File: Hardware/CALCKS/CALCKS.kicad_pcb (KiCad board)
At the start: 2 copper layers, 68 parts, among them J1 Conn_02x03_Counter_Clockwise, J2 USB_B_Micro, J3 Conn_01x01_Male, J4 Conn_01x01_Male, SW1 SW_Push_Dual, SW10 SW_Push_Dual, SW11 SW_Push_Dual, SW12 SW_Push_Dual, SW13 SW_Push_Dual, SW14 SW_Push_Dual, SW15 SW_Push_Dual, SW16 SW_Push_Dual, SW17 SW_Push_Dual, SW18 SW_Push_Dual, SW19 SW_Push_Dual, SW2 SW_Push_Dual, SW20 SW_Push_Dual, SW21 SW_Push_Dual, SW22 SW_Push_Dual, SW23 SW_Push_Dual, SW24 SW_Push_Dual, SW25 SW_Push_Dual, SW26 SW_Push_Dual, SW27 SW_Push_Dual, SW28 SW_Push_Dual, SW29 SW_Push_Dual, SW3 SW_Push_Dual, SW30 SW_Push_Dual, SW31 SW_Push_Dual, SW32 SW_Push_Dual, SW33 SW_Push_Dual, SW34 SW_Push_Dual, SW35 SW_Push_Dual, SW36 SW_Push_Dual, SW37 SW_Push_Dual, SW38 SW_Push_Dual, SW39 SW_Push_Dual, SW4 SW_Push_Dual, SW40 SW_Push_Dual, SW5 SW_Push_Dual, SW6 SW_Push_Dual, SW7 SW_Push_Dual, SW8 SW_Push_Dual, SW9 SW_Push_Dual, U1 ATmega1284-AU, U2 MCP73831-2-OT, U3 AT24CS64-SSHM, U4 74HC164, Y1 16MHz

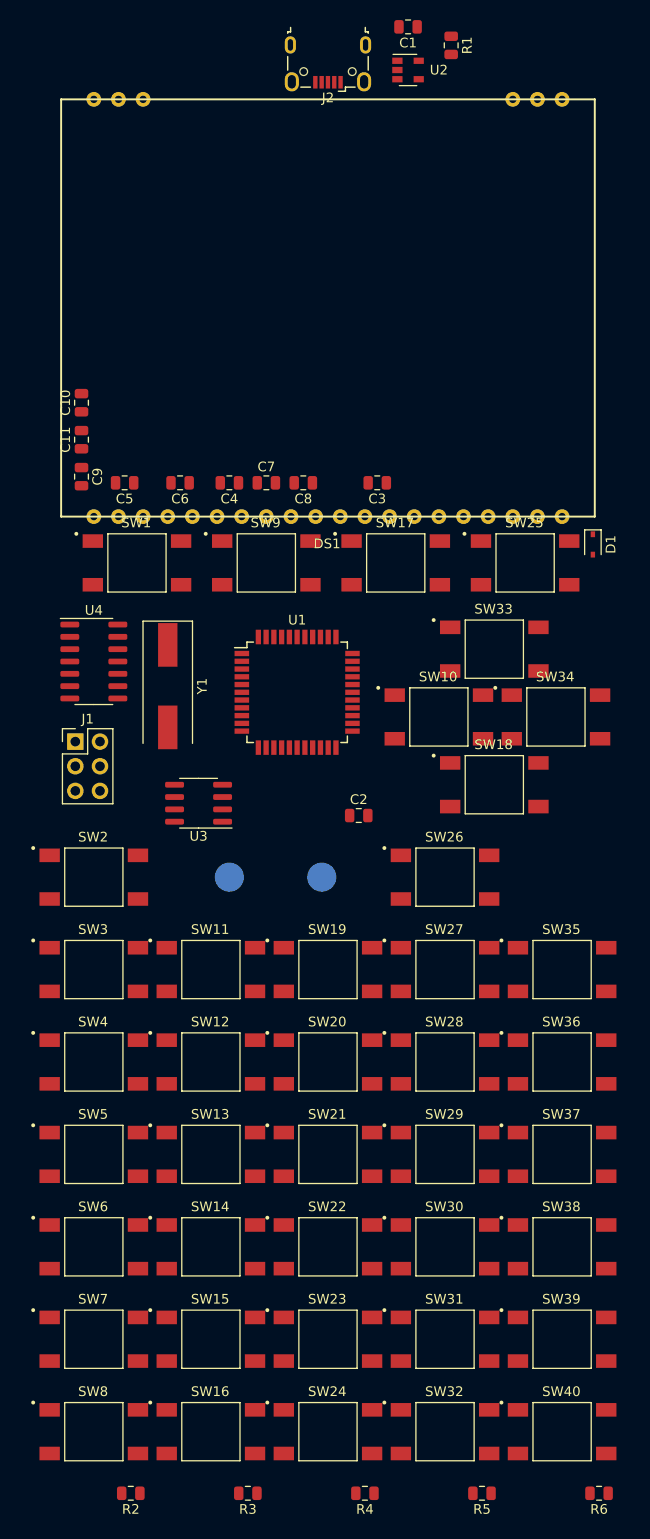
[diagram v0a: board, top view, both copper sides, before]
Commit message: PCB routing
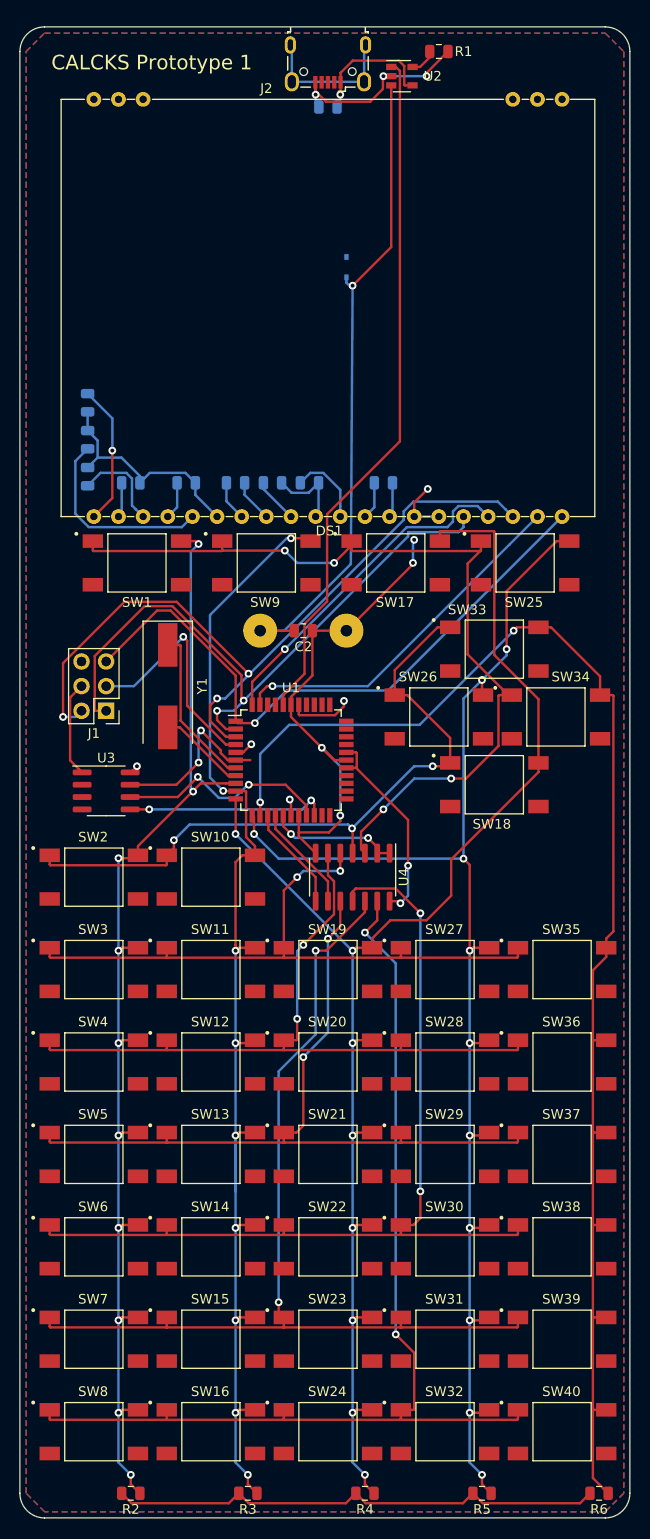
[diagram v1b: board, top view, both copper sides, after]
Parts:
- C1, C10, C11, C3, C4, C5, C6, C7, C8, C9, D1: moved to B.Cu
- J3, J4: footprint TestPoint:TestPoint_Pad_D3.0mm -> Connector_Wire:SolderWirePad_1x01_Drill1.2mm
- moved D1 38.2 mm to (100.3, 50.8)
- moved U4 34.7 mm to (101.0, 113.7), turned to 270 degrees
- moved SW10 28.7 mm to (86.4, 113.7)
- moved J3 28.1 mm to (100.3, 88.3)
- moved J4 26.2 mm to (91.4, 88.3)
- moved C2 19.9 mm to (95.9, 88.3), turned to 180 degrees
- moved SW26 16.5 mm to (109.9, 97.2)
- moved C1 11.7 mm to (98.4, 34.3)
- moved U3 9.61 mm to (75.6, 104.8), turned to 0 degrees
- moved C10 7.65 mm to (73.7, 72.4), turned to 270 degrees
- moved C9 7.65 mm to (73.7, 64.8), turned to 90 degrees
- moved U1 7.01 mm to (94.6, 101.6)
- moved J1 4.49 mm to (75.6, 96.5), turned to 180 degrees
- moved R1 1.42 mm to (109.9, 28.6), turned to 180 degrees
- moved U2 0.90 mm to (106.0, 31.1)
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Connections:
- net Net-(C2-Pad2) renamed +BATT
- C1 pad 2: GND -> Net-(C1-Pad2)
- C10 pad 1: GND -> -BATT
- C11 pad 1: GND -> -BATT
- C2 pad 1: GND -> -BATT
- C3 pad 1: GND -> -BATT
- C5 pad 1: GND -> -BATT
- C6 pad 1: GND -> -BATT
- C9 pad 1: GND -> -BATT
- DS1 pad 26: GND -> -BATT
- DS1 pad 33: GND -> -BATT
- J1 pad 4: GND -> -BATT
- J2 pad 5: GND -> Net-(C1-Pad2)
- J3 pad 1: GND -> -BATT
- R1 pad 1: GND -> Net-(C1-Pad2)
- R2 pad 2: GND -> -BATT
- R3 pad 2: GND -> -BATT
- R4 pad 2: GND -> -BATT
- R5 pad 2: GND -> -BATT
- R6 pad 2: GND -> -BATT
- U1 pad 18: GND -> -BATT
- U1 pad 28: GND -> -BATT
- U1 pad 39: GND -> -BATT
- U1 pad 6: GND -> -BATT
- U2 pad 2: GND -> Net-(C1-Pad2)
- U3 pad 1: GND -> -BATT
- U3 pad 2: GND -> -BATT
- U3 pad 3: GND -> -BATT
- U3 pad 4: GND -> -BATT
- U3 pad 7: GND -> -BATT
- U4 pad 7: GND -> -BATT
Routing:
- net -BATT: track 0.00 -> 159.5 mm, vias 0 -> 6
- net BTN_ROW3: track 0.00 -> 151.0 mm, vias 0 -> 8
- net BTN_ROW4: track 0.00 -> 143.7 mm, vias 0 -> 11
- net BTN_ROW5: track 0.00 -> 142.7 mm, vias 0 -> 2
- net BTN_ROW2: track 0.00 -> 128.7 mm, vias 0 -> 9
- net BTN_ROW1: track 0.00 -> 122.9 mm, vias 0 -> 10
- net Net-(SW16-Pad1): track 0.00 -> 109.6 mm, vias 0 -> 2
- net Net-(SW15-Pad1): track 0.00 -> 100.7 mm, vias 0 -> 2
- net Net-(SW14-Pad1): track 0.00 -> 96.1 mm, vias 0 -> 2
- net Net-(SW1-Pad1): track 0.00 -> 90.0 mm, vias 0 -> 4
- net Net-(SW13-Pad1): track 0.00 -> 80.3 mm, vias 0 -> 2
- net SCK: track 0.00 -> 78.6 mm, vias 0 -> 3
- net Net-(SW12-Pad1): track 0.00 -> 75.7 mm, vias 0 -> 2
- net BATT_STATUS: track 0.00 -> 71.4 mm
- net Net-(SW10-Pad1): track 0.00 -> 70.8 mm, vias 0 -> 3
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- added copper zone on F.Cu, net -BATT
- added copper zone on B.Cu, net VCC
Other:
- board outline added: 62.9 x 153.7 mm
- board text added: "CALCKS Prototype 1"
